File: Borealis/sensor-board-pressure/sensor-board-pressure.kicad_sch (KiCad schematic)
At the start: 5 parts, among them J2 Conn_01x03_Pin (data connecti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, J5 Conn_01x03_Pin (power connect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

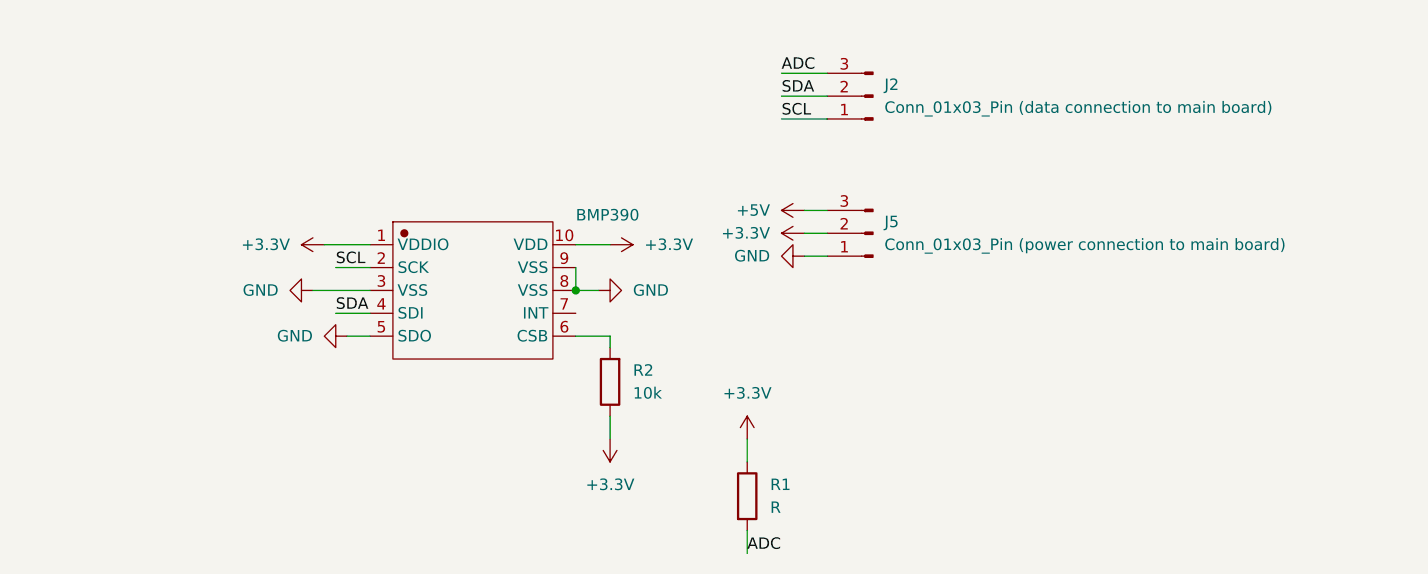
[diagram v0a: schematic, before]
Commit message: Fixed a few things
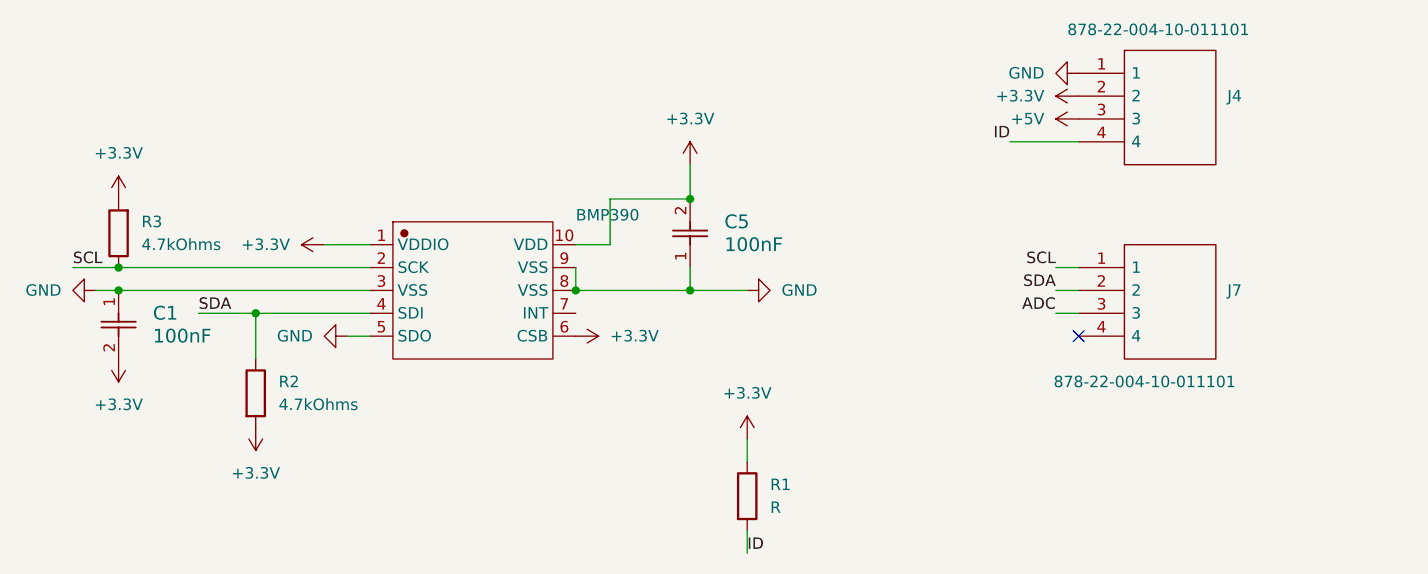
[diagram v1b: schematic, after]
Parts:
- removed J2: Conn_01x03_Pin (data connection to main board), batteryholder:1x03 2.3 pitch, symbol Connector:Conn_01x03_Pin
- removed J5: Conn_01x03_Pin (power connection to main board), batteryholder:1x03 2.3 pitch, symbol Connector:Conn_01x03_Pin
- added C1, C5: 100nF, BOREALIS:CAPC17595_95N_KEM, symbol 2026-01-23_05-30-51:C0603C104K5RACTU
- added J4, J7: 878-22-004-10-011101, BOREALIS:8782200410011101, symbol 878-22-004-10-011101:878-22-004-10-011101
- added R3: 4.7kOhms, Resistor_SMD:R_0805_2012Metric, symbol Device:R
- R2: value 10k -> 4.7kOhms
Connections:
- net +3.3V: now also BMP390.6 (CSB), R2.2, C1.2, C5.2, J4.2, R3.2; no longer R2.1
- net +5V: now also J4.3
- net ADC: now also J7.3; no longer R1.2
- net GND: now also C1.1, C5.1, J4.1
- net SCL: now also J7.1, R3.1
- net SDA: now also R2.1, J7.2
- new net ID: J4.4, R1.2
- no-connect marks 0 -> 1
